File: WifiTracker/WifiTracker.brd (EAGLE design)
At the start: 158.7 x 101.3 mm, 24 parts, among them Y1 16MHz

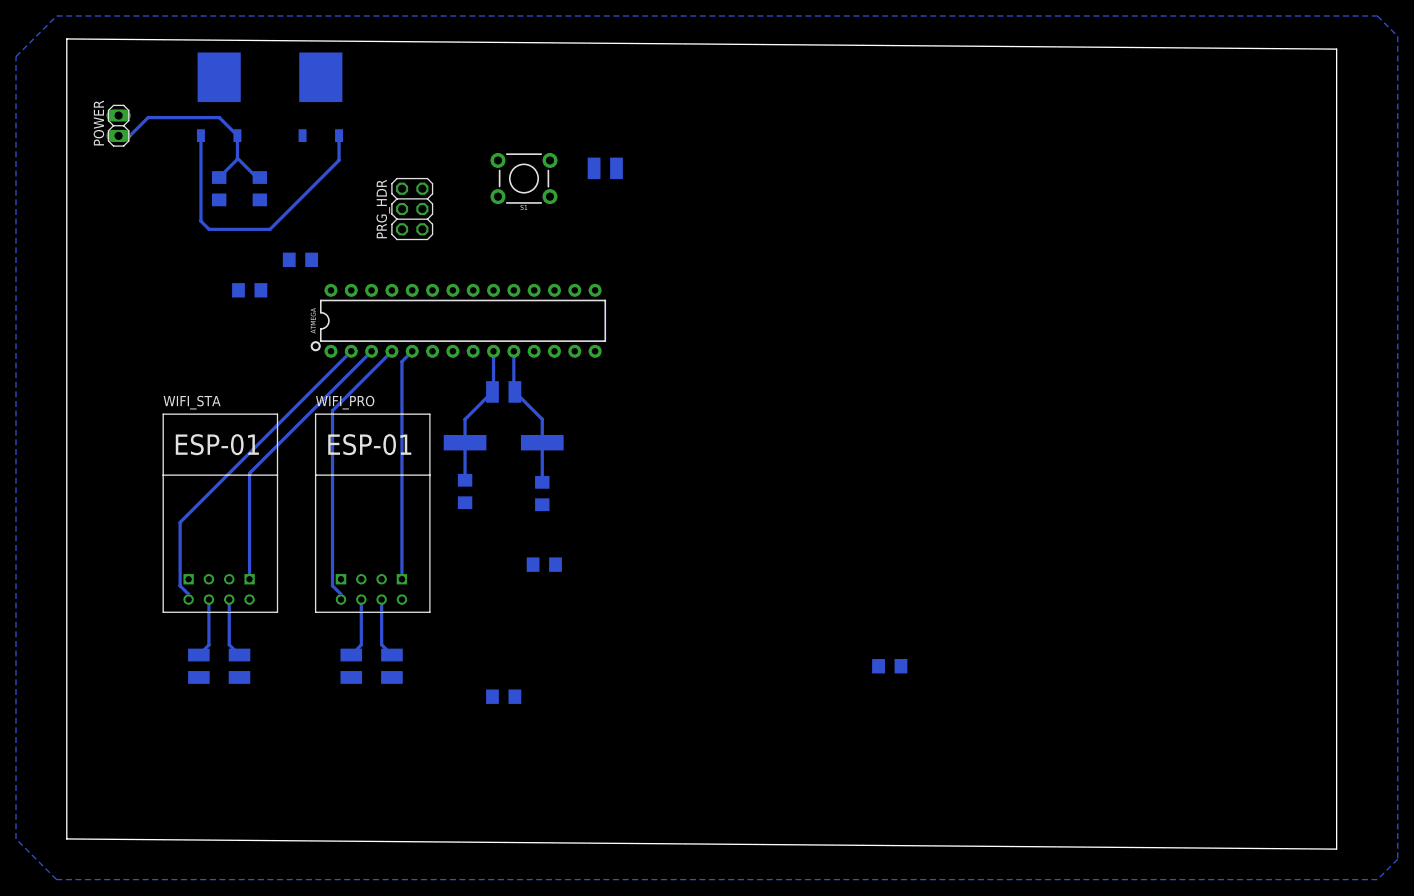
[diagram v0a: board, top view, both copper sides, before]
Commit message: Rev 1
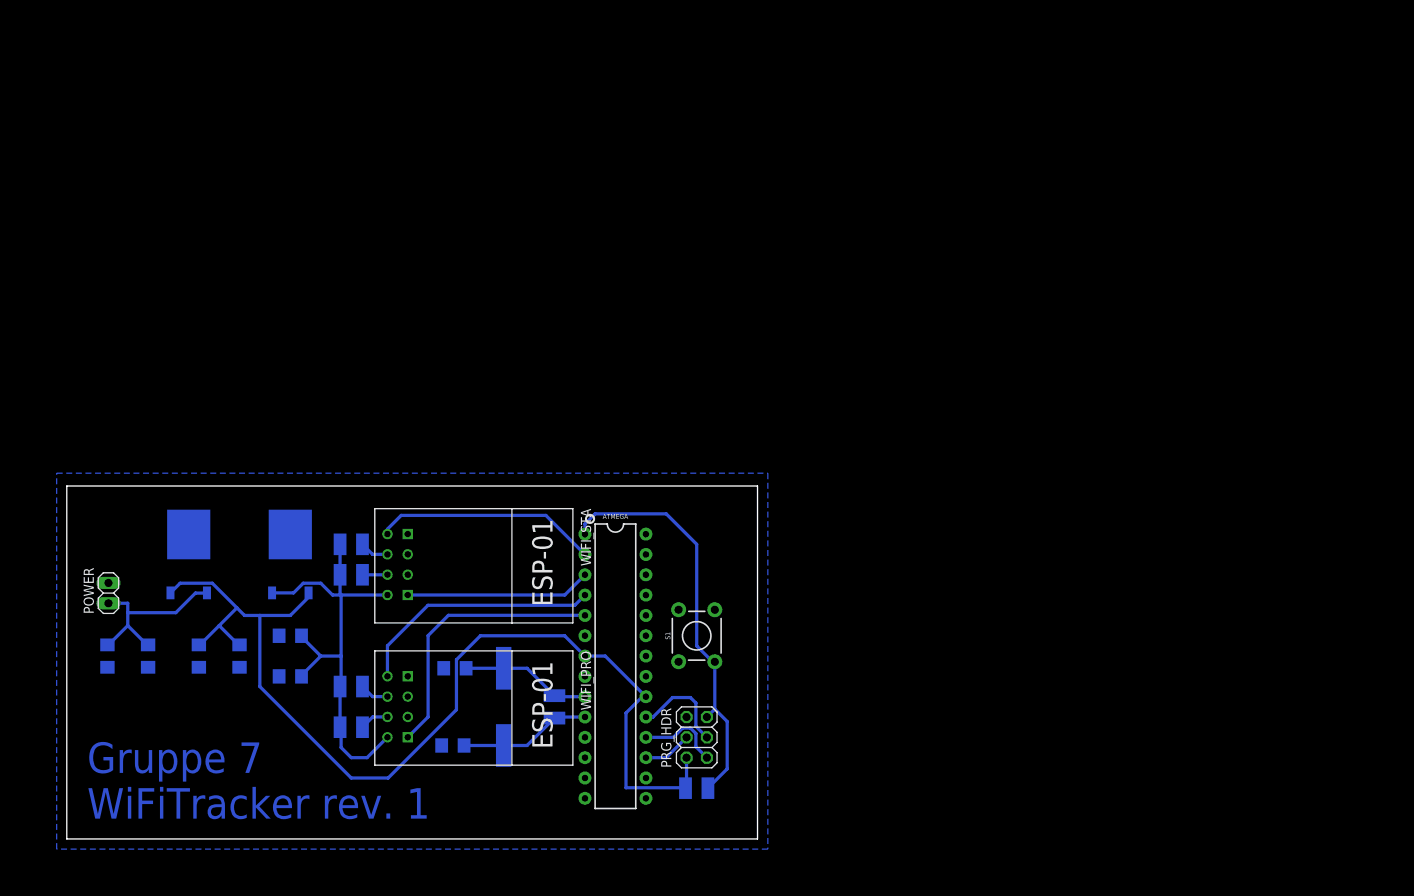
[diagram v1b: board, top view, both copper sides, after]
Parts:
- removed C3: 0.1uF, SparkFun-Capacitors:1206
- moved R6 78.3 mm to (78.7, 6.35), turned to 180 degrees
- moved PRG_HDR 75.0 mm to (78.7, 12.7)
- moved C6 74.9 mm to (27.9, 20.3)
- moved C4 61.4 mm to (5.08, 22.9)
- moved S1 61.1 mm to (78.7, 25.4), turned to 90 degrees
- moved C7 59.1 mm to (10.2, 22.9)
- moved POWER 58.4 mm to (5.21, 30.7)
- moved 3V_REG 57.3 mm to (27.9, 35.6)
- moved 5V_REG 57.3 mm to (15.2, 35.6)
- moved C5 50.1 mm to (21.6, 22.9), turned to 270 degrees
- moved ATMEGA 47.2 mm to (68.6, 21.6), turned to 270 degrees
- moved C8 46.2 mm to (16.5, 22.9), turned to 270 degrees
- moved R4 39.9 mm to (61.0, 16.5), turned to 90 degrees
- moved C2 33.4 mm to (48.3, 11.7), turned to 180 degrees
- moved Y1 33.0 mm to (54.6, 16.5), turned to 90 degrees
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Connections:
- net N$1 renamed STA_CH_PD
- net N$2 renamed STA_RST
- net N$3 renamed PRO_CH_PD
- net N$4 renamed PRO_RST
- net 5VCC: no longer C3.1
- net GND: no longer C3.2
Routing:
- net 5VCC: track 35.4 -> 131.6 mm
- net 3VCC: track 0.00 -> 58.5 mm
- net ATMEGA_RESET: track 0.00 -> 52.0 mm
- net SCK: track 0.00 -> 12.4 mm
- net STA_TXD: track 40.3 -> 28.0 mm
- net STA_RXD: track 34.8 -> 23.2 mm
- net MISO: track 0.00 -> 10.6 mm
- net MOSI: track 0.00 -> 6.13 mm
- net PRO_RXD: track 29.0 -> 34.4 mm
- net STA_RST: track 7.46 -> 3.13 mm
- net STA_CH_PD: track 7.45 -> 3.64 mm
- net PRO_RST: track 7.46 -> 3.65 mm
- net PRO_CH_PD: track 7.45 -> 3.64 mm
- net PRO_TXD: track 34.6 -> 31.1 mm
- net VIN: track 26.7 -> 23.6 mm
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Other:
- board size 158.7 x 101.3 mm -> 86.3 x 44.1 mm
- board text added: "Gruppe 7 WiFiTracker rev. 1"
